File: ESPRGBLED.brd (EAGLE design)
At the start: 21.3 x 27 mm, 23 parts

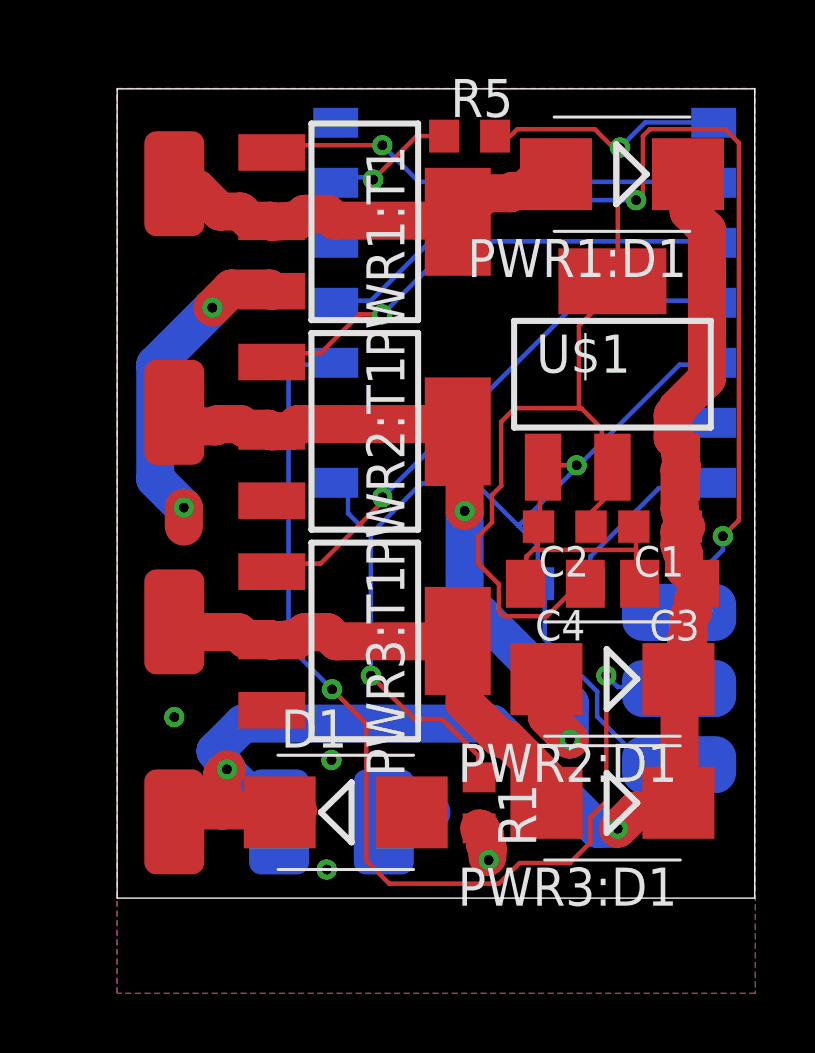
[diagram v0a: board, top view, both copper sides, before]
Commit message: smd
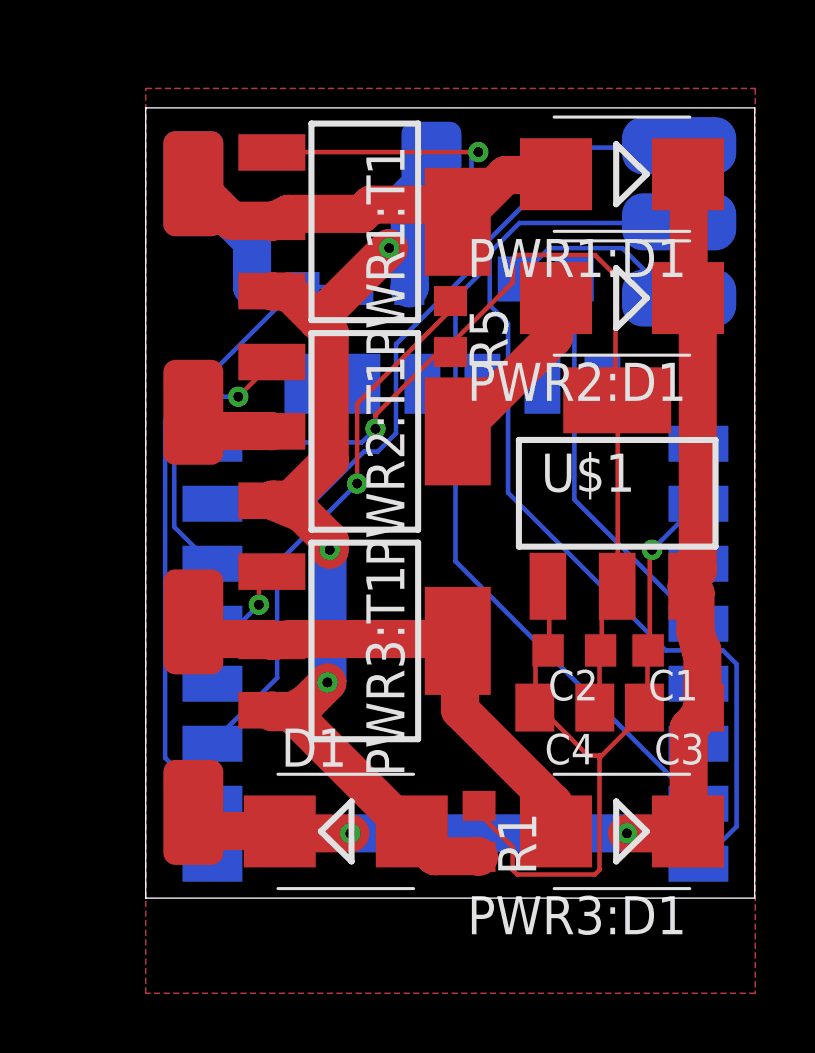
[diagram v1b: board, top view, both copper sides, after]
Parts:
- removed U$2: ESP8266, ESP8266:ESP-03
- added MDL1: (no value), ESP8266-ESP12E:ESP8266-ESP12E
- added R3: 100k, rcl:R0603
- added R4: 10k, rcl:R0603
- R2: device rcl:R0603 -> rcl:R0805
- moved U$8 21.6 mm to (10.5, 27.3)
- moved U$7 21.5 mm to (2.54, 27.0)
- moved U$3 15.6 mm to (18.7, 25.7)
- moved PWR2:D1 12.7 mm to (16.8, 23.2)
- moved R2 10.2 mm to (14.3, 23.8)
- moved R5 6.38 mm to (11.1, 22.2), turned to 270 degrees
- moved C1 4.15 mm to (18.6, 11.4)
- moved C2 4.14 mm to (15.2, 11.4)
- moved C4 4.14 mm to (14.9, 9.53)
- moved C3 4.13 mm to (18.6, 9.53)
- moved U$1 3.97 mm to (16.7, 16.7)
- moved PWR3:D1 1.00 mm to (16.8, 5.40)
- moved R1 0.95 mm to (12.1, 5.40)
- moved U$9 0.71 mm to (2.54, 6.03)
- moved U$4 0.64 mm to (2.54, 27.0)
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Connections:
- new net N$10: MDL1.2, R3.1, R4.2
- net +12V: now also R3.2
- net DGND: now also MDL1.10, MDL1.9; no longer U$2.GND, U$2.GPIO15
- net GND: now also R4.1
- net N$11: now also MDL1.3; no longer U$2.CH_PD
- net N$2: now also MDL1.5; no longer U$2.GPIO13
- net N$3: now also MDL1.6; no longer U$2.GPIO12
- net N$6: now also MDL1.7; no longer U$2.GPIO14
- net N$7: now also MDL1.15; no longer U$2.URXD
- net N$8: now also MDL1.16; no longer U$2.UTXD
- net N$9: now also MDL1.12; no longer U$2.GPIO0
- net VCC: now also MDL1.8; no longer U$2.VCC
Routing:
- net N$10: track 0.00 -> 21.8 mm
- net GND: track 13.8 -> 35.1 mm, vias 6 -> 3
- net N$2: track 18.6 -> 3.10 mm
- net N$4: track 24.1 -> 8.74 mm, vias 2 -> 0
- net N$11: track 4.32 -> 18.0 mm
- net N$6: track 15.3 -> 24.5 mm
- net DGND: track 48.9 -> 40.2 mm, vias 2 -> 1
- net N$9: track 6.03 -> 13.2 mm
- net N$3: track 16.4 -> 9.36 mm
- net +12V: track 49.6 -> 43.7 mm
- net N$8: track 35.7 -> 32.2 mm, vias 2 -> 0
- net N$7: track 33.6 -> 30.3 mm, vias 2 -> 0
- net VCC: track 35.1 -> 32.0 mm
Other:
- board size 21.3 x 27 mm -> 20.3 x 26.3 mm

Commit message: through hole
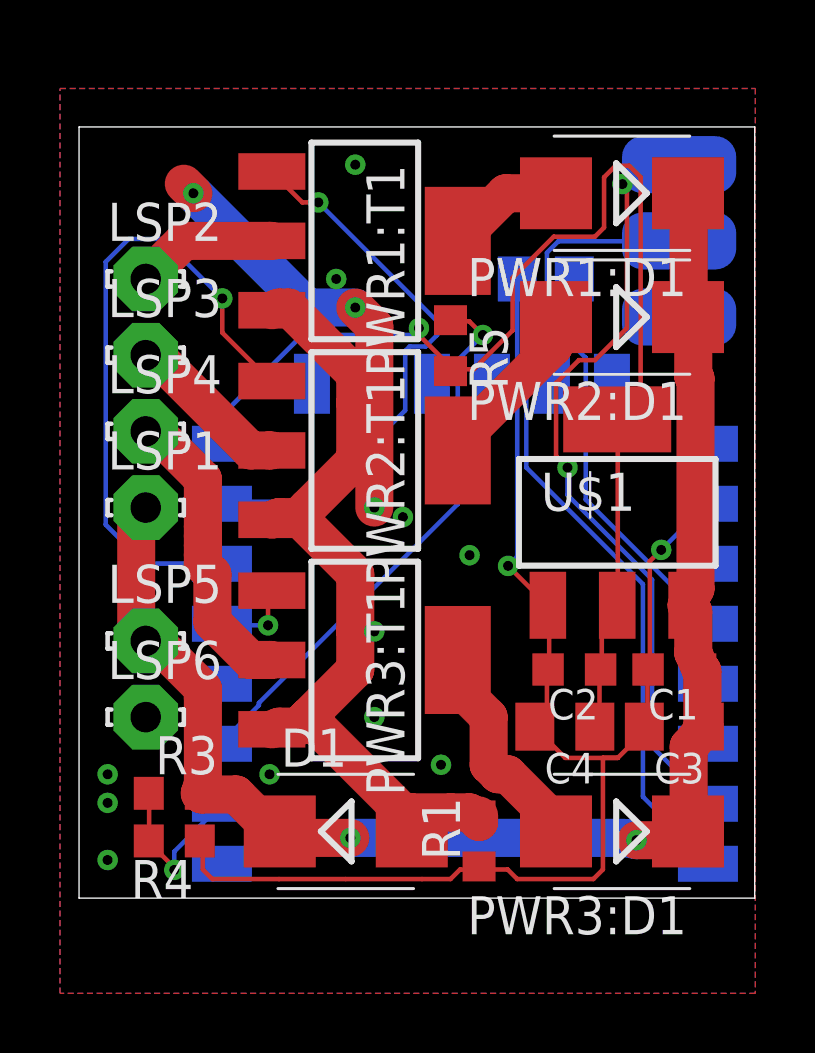
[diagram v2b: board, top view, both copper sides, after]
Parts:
- removed U$4, U$5, U$6, U$7, U$8, U$9: CON1, Fabian:CON1HP
- added LSP1, LSP2, LSP3, LSP4, LSP5, LSP6: LSP10, solpad:LSP10
- moved R4 19.7 mm to (1.91, 5.08), flipped to the top, turned to 180 degrees
- moved R3 17.2 mm to (1.91, 6.67), flipped to the top
- moved PWR1:T1 0.64 mm to (8.26, 25.1)
- moved PWR2:T1 0.64 mm to (8.26, 18.1)
- moved R5 0.64 mm to (11.1, 21.6)
- moved U$3 0.64 mm to (18.7, 25.1)
- moved C1 0.63 mm to (18.6, 10.8)
- moved C2 0.63 mm to (15.2, 10.8)
- moved C3 0.63 mm to (18.6, 8.89)
- moved C4 0.63 mm to (14.9, 8.89)
- moved PWR3:T1 0.63 mm to (8.26, 11.1)
- moved PWR1:D1 0.63 mm to (16.8, 26.7)
- moved PWR2:D1 0.63 mm to (16.8, 22.5)
- moved U$1 0.63 mm to (16.7, 16.0)
- moved MDL1 0.32 mm to (3.49, 20.3)
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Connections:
- net +12V: now also LSP1.MP, LSP5.MP; no longer U$7.P$1, U$9.P$1
- net DGND: now also R4.1
- net GND: now also LSP6.MP; no longer R4.1, U$8.P$1
- net N$1: now also LSP2.MP; no longer U$4.P$1
- net N$4: now also LSP3.MP; no longer U$5.P$1
- net N$5: now also LSP4.MP; no longer U$6.P$1
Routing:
- net DGND: track 40.2 -> 57.0 mm, vias 1 -> 2
- net N$10: track 21.8 -> 5.77 mm, vias 0 -> 1
- net N$3: track 9.36 -> 21.7 mm
- net VCC: track 32.0 -> 40.9 mm
- net GND: track 35.1 -> 42.5 mm, vias 3 -> 14
- net +12V: track 43.7 -> 49.5 mm
- net N$6: track 24.5 -> 18.7 mm
- net N$1: track 13.6 -> 8.66 mm
- net N$8: track 32.2 -> 28.4 mm
- net N$7: track 30.3 -> 27.0 mm, vias 0 -> 2
- net N$4: track 8.74 -> 11.3 mm
- net N$5: track 16.9 -> 17.7 mm
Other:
- board size 20.3 x 26.3 mm -> 22.5 x 25.7 mm
